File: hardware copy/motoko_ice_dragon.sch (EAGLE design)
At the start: 119 parts, among them IC2 LM2937, Q1 8MHz, Q10 20mA/30V, Q11 20mA/30V, Q2 BSS138TOP, Q3 BSS138TOP, Q4 20mA/30V, Q5 20mA/30V, Q6 20mA/30V, Q7 20mA/30V, Q8 20mA/30V, Q9 20mA/30V, U1 MP6540HA, U2 STM32_STM32F722XX, U3 MP6540HA

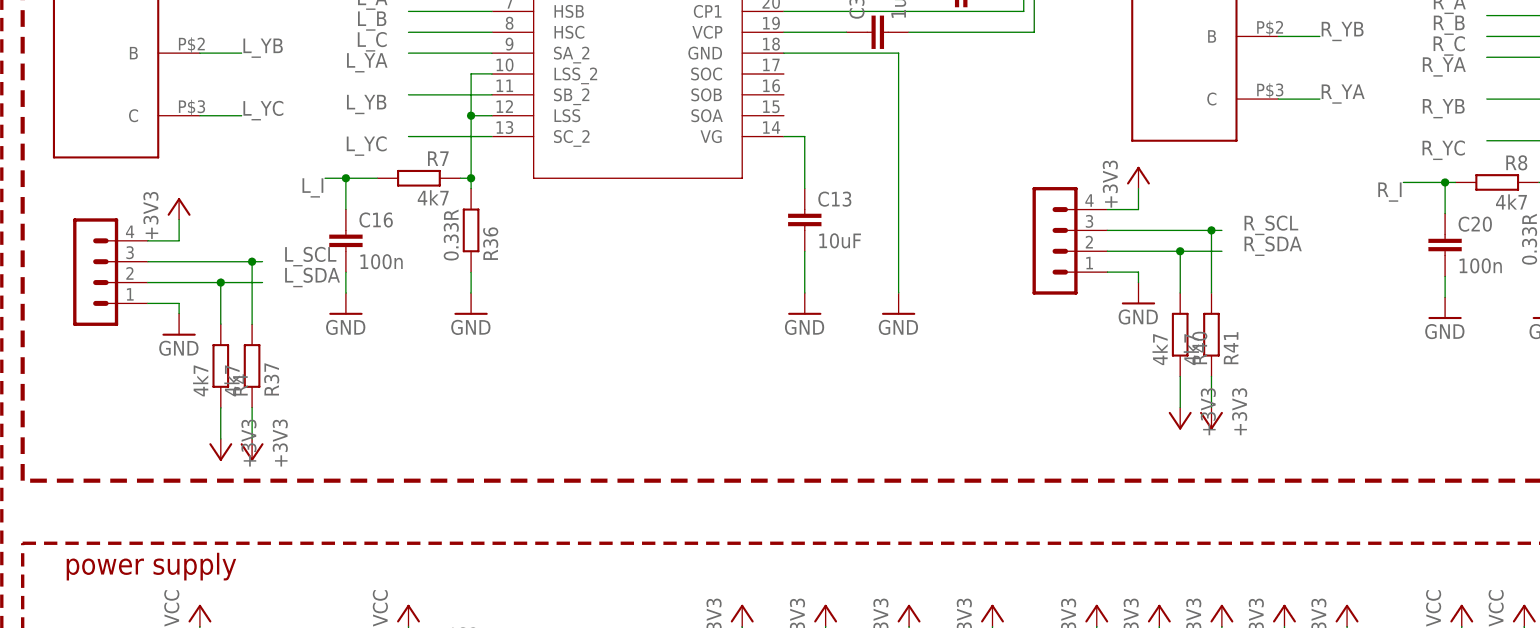
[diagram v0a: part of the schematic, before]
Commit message: main board
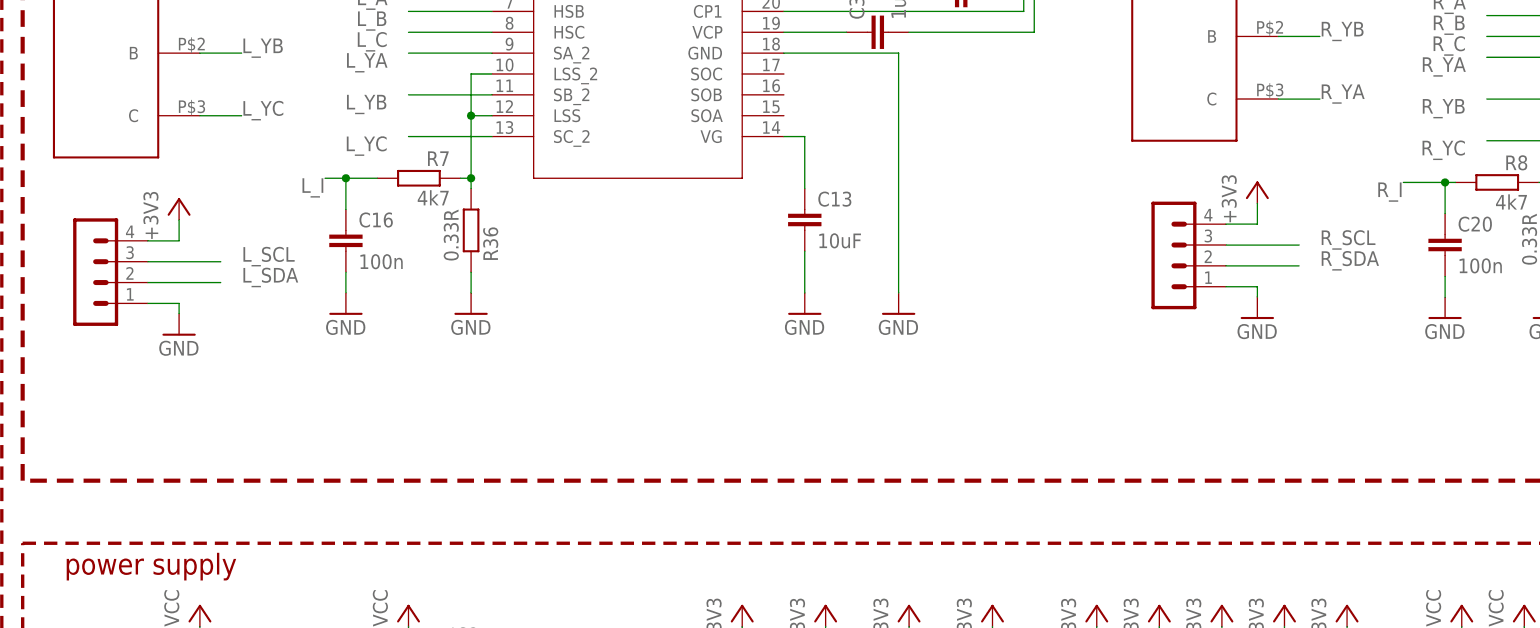
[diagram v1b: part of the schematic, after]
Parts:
- removed L_ENCODER1: (no value), con-lstb:MA04-1
- removed R37, R4, R40, R41: 4k7, resistor:R-EU_M0805
- added R_ENCODER: (no value), con-lstb:MA04-1
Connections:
- net +3V3: now also R_ENCODER.4; no longer L_ENCODER1.4, R37.1, R4.1, R40.1, R41.1
- net GND: now also R_ENCODER.1; no longer L_ENCODER1.1
- net L_SCL: no longer R37.2
- net L_SDA: no longer R4.2
- net R_SCL: now also R_ENCODER.3; no longer L_ENCODER1.3, R41.2
- net R_SDA: now also R_ENCODER.2; no longer L_ENCODER1.2, R40.2

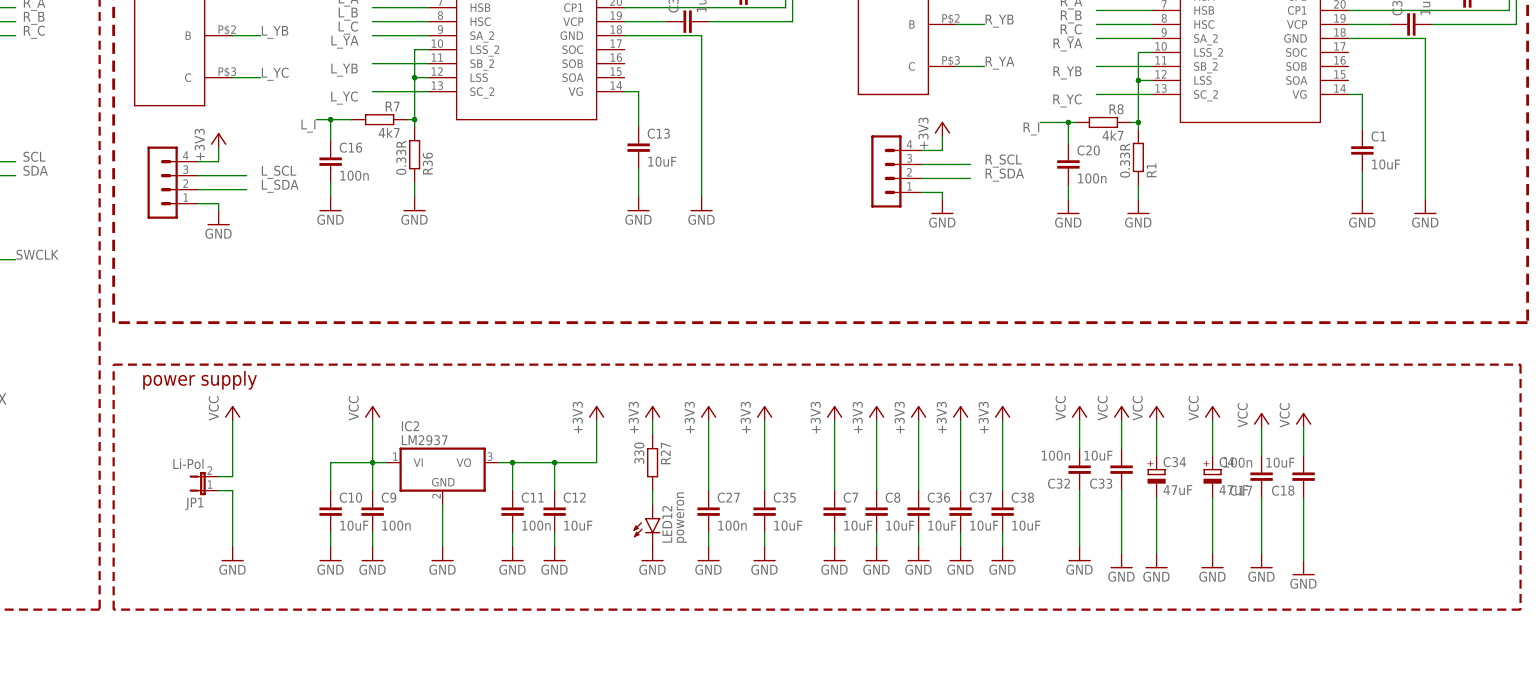
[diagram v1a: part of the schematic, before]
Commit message: main board
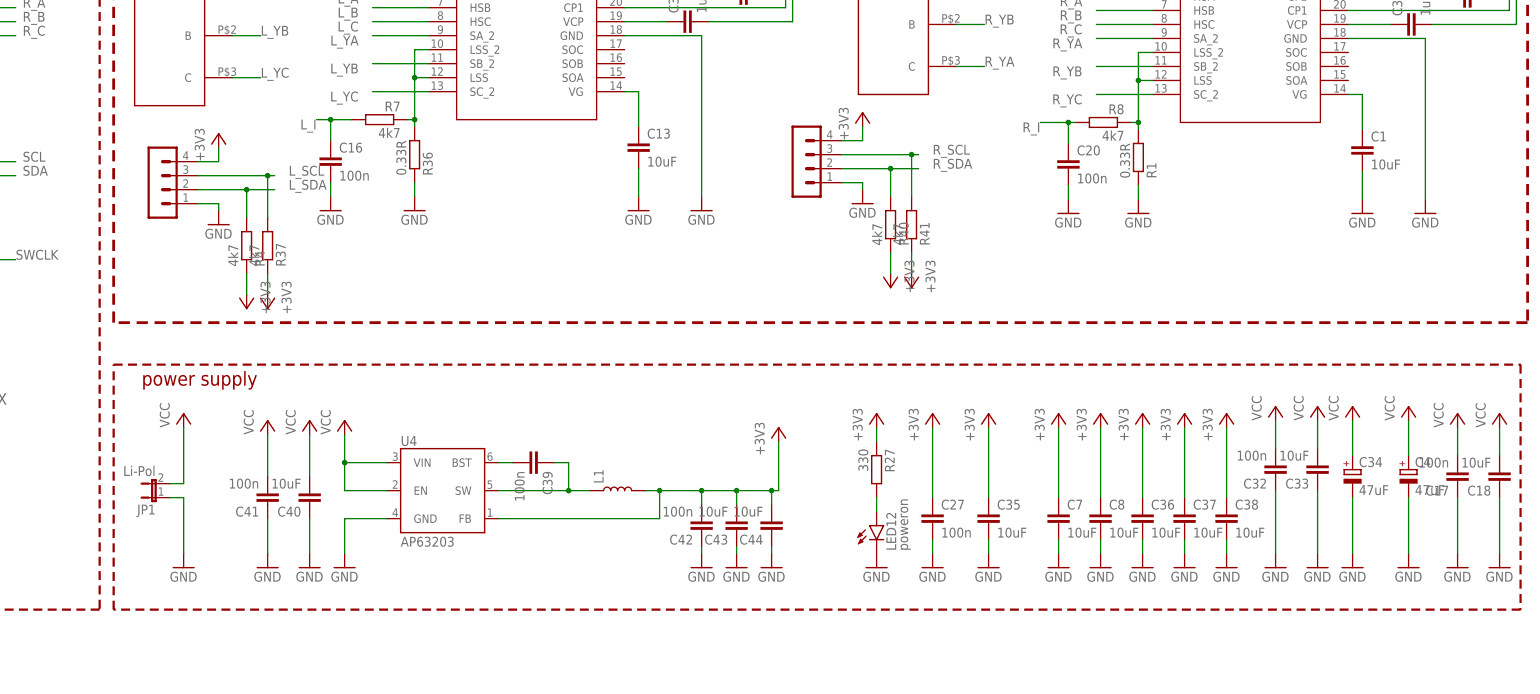
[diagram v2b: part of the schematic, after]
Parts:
- removed C10, C12: 10uF, resistor:C-EUC0805
- removed C11, C9: 100n, resistor:C-EUC0805
- removed IC2: LM2937, linear:LM2937
- removed R_ENCODER: (no value), con-lstb:MA04-1
- added C39, C41, C42: 100n, resistor:C-EUC0805
- added C40, C43, C44: 10uF, resistor:C-EUC0805
- added L1: 4.7uH, TYS50204R7N-10, SparkFun-Coils:INDUCTOR-CR54-3.3UH
- added L_ENCODER1: (no value), con-lstb:MA04-1
- added R37, R4, R40, R41: 4k7, resistor:R-EU_M0805
- added U4: AP63203, SparkFun-IC-Power:AP63203
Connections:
- new net N$22: C39.2, U4.BST
- new net N$26: C39.1, L1.1, U4.SW
- net +3V3: now also C42.2, C43.2, C44.2, L1.2, L_ENCODER1.4, R37.1, R4.1, R40.1, R41.1, U4.FB; no longer C11.1, C12.1, IC2.VO, R_ENCODER.4
- net GND: now also C40.1, C41.1, C42.1, C43.1, C44.1, L_ENCODER1.1, U4.GND; no longer C10.2, C11.2, C12.2, C9.2, IC2.GND, R_ENCODER.1
- net L_SCL: now also R37.2
- net L_SDA: now also R4.2
- net R_SCL: now also L_ENCODER1.3, R41.2; no longer R_ENCODER.3
- net R_SDA: now also L_ENCODER1.2, R40.2; no longer R_ENCODER.2
- net VCC: now also C40.2, C41.2, U4.EN, U4.VIN; no longer C10.1, C9.1, IC2.VI
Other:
- moved on the sheet: C17, C18, C27, C32, C33, C34, C35, C36, C37, C38, C4, C7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
